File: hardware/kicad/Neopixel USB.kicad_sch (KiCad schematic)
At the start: 12 parts, among them U1 ATtiny85-20S

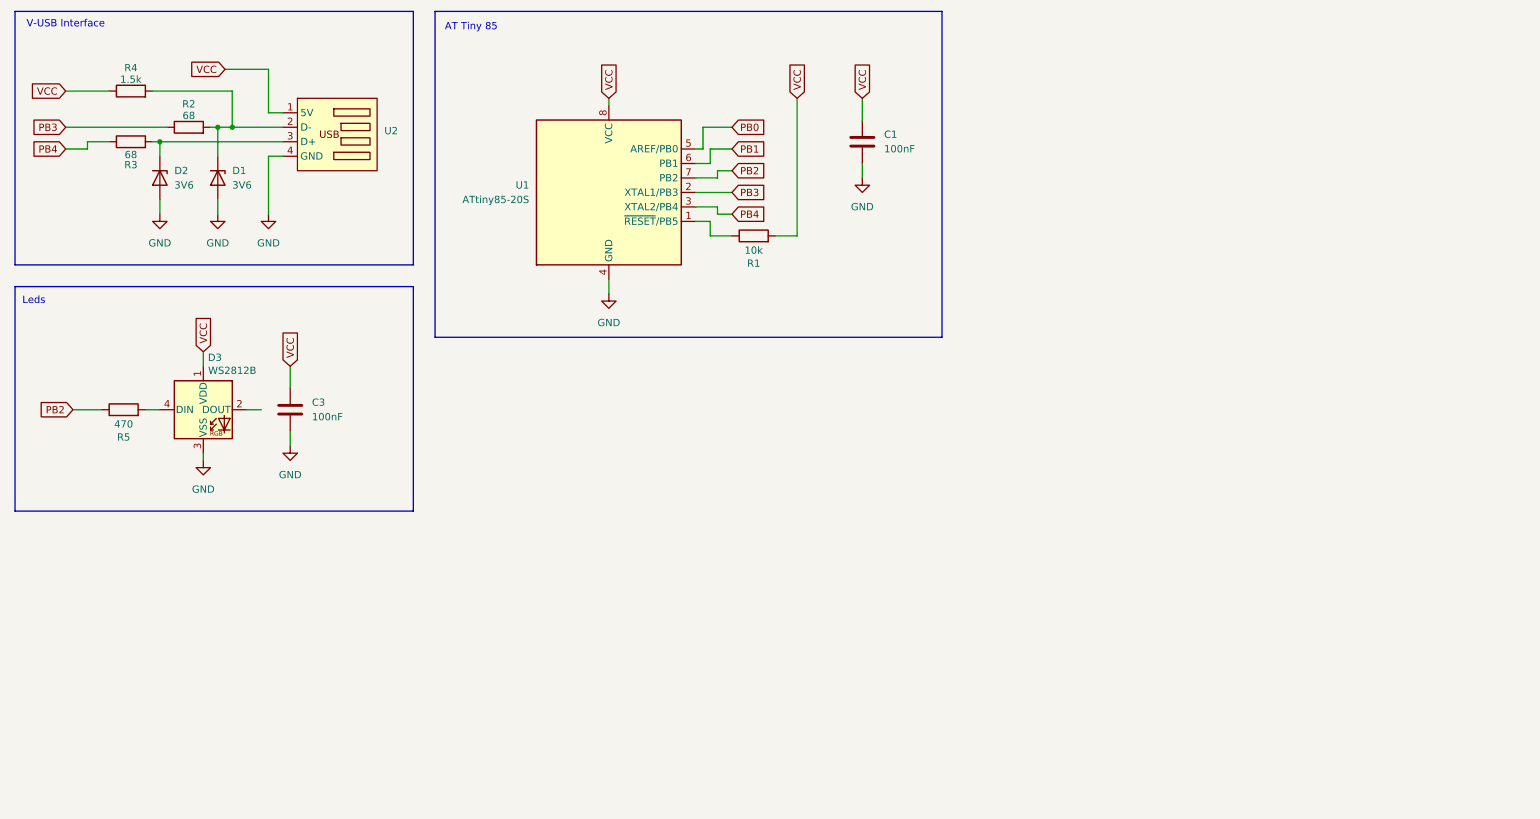
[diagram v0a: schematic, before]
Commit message: Mise à jour du schema
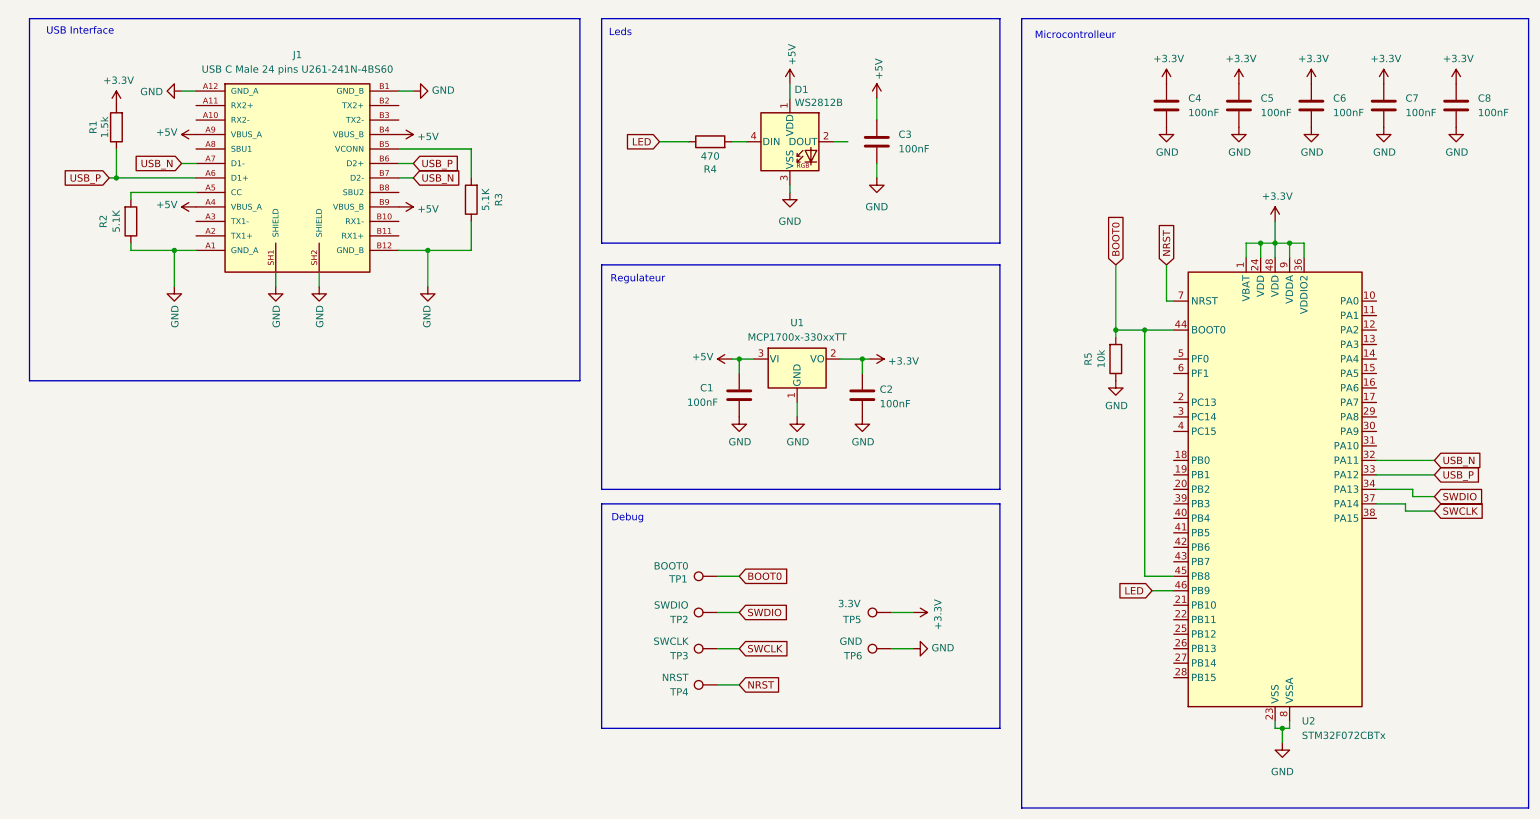
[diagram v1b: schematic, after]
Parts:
- removed D1, D2: 3V6, Diode_SMD:D_SOD-123, symbol Device:D_Zener
- removed R4: 1.5k, Resistor_SMD:R_0603_1608Metric_Pad0.98x0.95mm_HandSolder, symbol Device:R
- removed U1: ATtiny85-20S, Package_SO:SOIC-8_5.3x5.3mm_P1.27mm, symbol MCU_Microchip_ATtiny:ATtiny85-20S
- removed U2: ~, arthur:USB A Male PCB, symbol arthur:PCB_USB_typeA_Male
- added C2, C4, C5, C6, C7, C8: 100nF, Capacitor_SMD:C_0603_1608Metric, symbol Device:C
- added J1: USB C Male 24 pins U261-241N-4BS60, arthur:USB-C male 24 pins XKB_U261-241N-4BS60, symbol arthur:USB C Male 24 pins U261-241N-4BS60
- added R5: 10k, Resistor_SMD:R_0603_1608Metric, symbol Device:R
- added TP1: BOOT0, arthur:TestPoint_Pad_D1.0mm_1, symbol Connector:TestPoint
- added TP2: SWDIO, arthur:TestPoint_Pad_D1.0mm_1, symbol Connector:TestPoint
- added TP3: SWCLK, arthur:TestPoint_Pad_D1.0mm_1, symbol Connector:TestPoint
- added TP4: NRST, arthur:TestPoint_Pad_D1.0mm_1, symbol Connector:TestPoint
- added TP5: 3.3V, arthur:TestPoint_Pad_D1.0mm_1, symbol Connector:TestPoint
- added TP6: GND, arthur:TestPoint_Pad_D1.0mm_1, symbol Connector:TestPoint
- added U1: MCP1700x-330xxTT, Package_TO_SOT_SMD:SOT-23, symbol Regulator_Linear:MCP1700x-330xxTT
- added U2: STM32F072CBTx, Package_QFP:LQFP-48_7x7mm_P0.5mm, symbol MCU_ST_STM32F0:STM32F072CBTx
- C1, C3: footprint Capacitor_SMD:C_0603_1608Metric_Pad1.08x0.95mm_HandSolder -> Capacitor_SMD:C_0603_1608Metric
- R1: value 10k -> 1.5k; footprint Resistor_SMD:R_0603_1608Metric_Pad0.98x0.95mm_HandSolder -> Resistor_SMD:R_0603_1608Metric; LCSC C25804 -> C22843
- R2, R3: value 68 -> 5.1K; footprint Resistor_SMD:R_0603_1608Metric_Pad0.98x0.95mm_HandSolder -> Resistor_SMD:R_0603_1608Metric; LCSC C27592 -> C23186
- R4: renamed from R5; footprint Resistor_SMD:R_0603_1608Metric_Pad0.98x0.95mm_HandSolder -> Resistor_SMD:R_0603_1608Metric
- renumbered D3 to D1
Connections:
- net PB3 is gone; now on net GND: R2.1
- net PB4 is gone; now on net GND: R3.1
- net GND: now also C2.2, C4.2, C5.2, C6.2, C7.2, C8.2, J1.A1 (GND_A), J1.A12 (GND_A), J1.B1 (GND_B), J1.B12 (GND_B), J1.SH1 (SHIELD), J1.SH2 (SHIELD), R5.1, TP6.1, U1.1 (GND), U2.23 (VSS), U2.35 (VSS), U2.47 (VSS), U2.8 (VSSA)
- net at R2.2: now also J1.A5 (CC)
- net USB_P: now reaches R1.1
- net USB_P: now also J1.A6 (D1+), J1.B6 (D2+), U2.33 (PA12)
- net at R3.2: now also J1.B5 (VCONN)
- net PB2 renamed LED
- net LED: now also U2.46 (PB9)
- net VCC renamed +5V
- net +5V: now also J1.A4 (VBUS_A), J1.A9 (VBUS_A), J1.B4 (VBUS_B), J1.B9 (VBUS_B), U1.3 (VI); no longer R1.2
- new net +3.3V: C2.1, C4.1, C5.1, C6.1, C7.1, C8.1, R1.2, TP5.1, U1.2 (VO), U2.1 (VBAT), U2.24 (VDD), U2.36 (VDDIO2), U2.48 (VDD), U2.9 (VDDA)
- new net BOOT0: R5.2, TP1.1, U2.44 (BOOT0), U2.45 (PB8)
- new net NRST: TP4.1, U2.7 (NRST)
- new net SWCLK: TP3.1, U2.37 (PA14)
- new net SWDIO: TP2.1, U2.34 (PA13)
- new net USB_N: J1.A7 (D1-), J1.B7 (D2-), U2.32 (PA11)
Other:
- note added: "Debug"
- note added: "Microcontrolleur"
- note added: "Regulateur"
- note added: "USB Interface"
- note removed: "AT Tiny 85"
- note removed: "V-USB Interface"
- moved on the sheet: C3, D1, R4
